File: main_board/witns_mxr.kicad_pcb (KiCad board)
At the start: 2 copper layers, 19 x 110 mm, 30 parts, among them J101 CH1, J102 CH2, J103 CH3, J104 CH4, J105 OUT, J106 POWER, U1 TL072

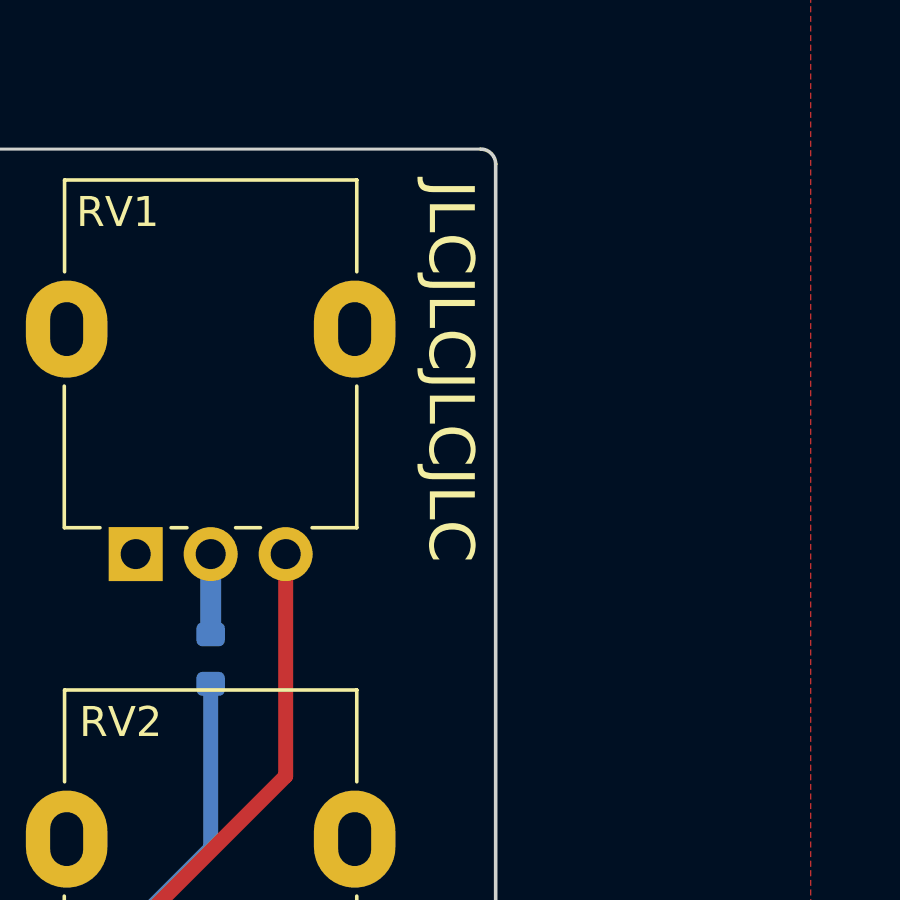
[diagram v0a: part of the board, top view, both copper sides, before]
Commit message: JLC mark
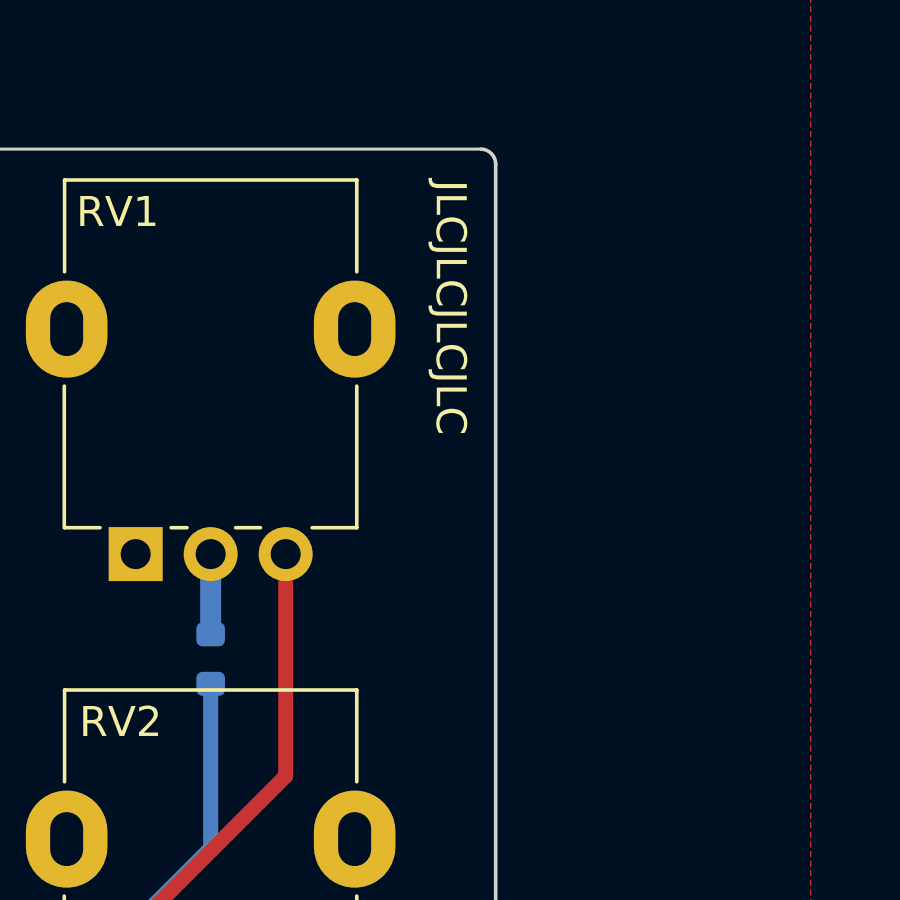
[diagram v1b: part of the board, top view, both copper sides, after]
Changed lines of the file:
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@@
   (gr_line (start 41.5 153.5) (end 50.5 153.5) (layer "B.SilkS") (width 0.8))
   (gr_text "JLCJLCJLCJLC" (at 58 46.03 270) (layer "F.SilkS")
-    (effects (font (size 1.5 1.5) (thickness 0.3)) (justify left))
+    (effects (font (size 1 1) (thickness 0.15)) (justify left))
   )
   (gr_text "WITNS\nMXR\nv1.0\nLF" (at 40.8 148.3) (layer "F.SilkS")
